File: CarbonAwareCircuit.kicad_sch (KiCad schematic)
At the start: 3 parts, among them J1 USB_C_Receptacle_PowerOnly_6P, U1 LD1117V33, U2 ESP32-C3

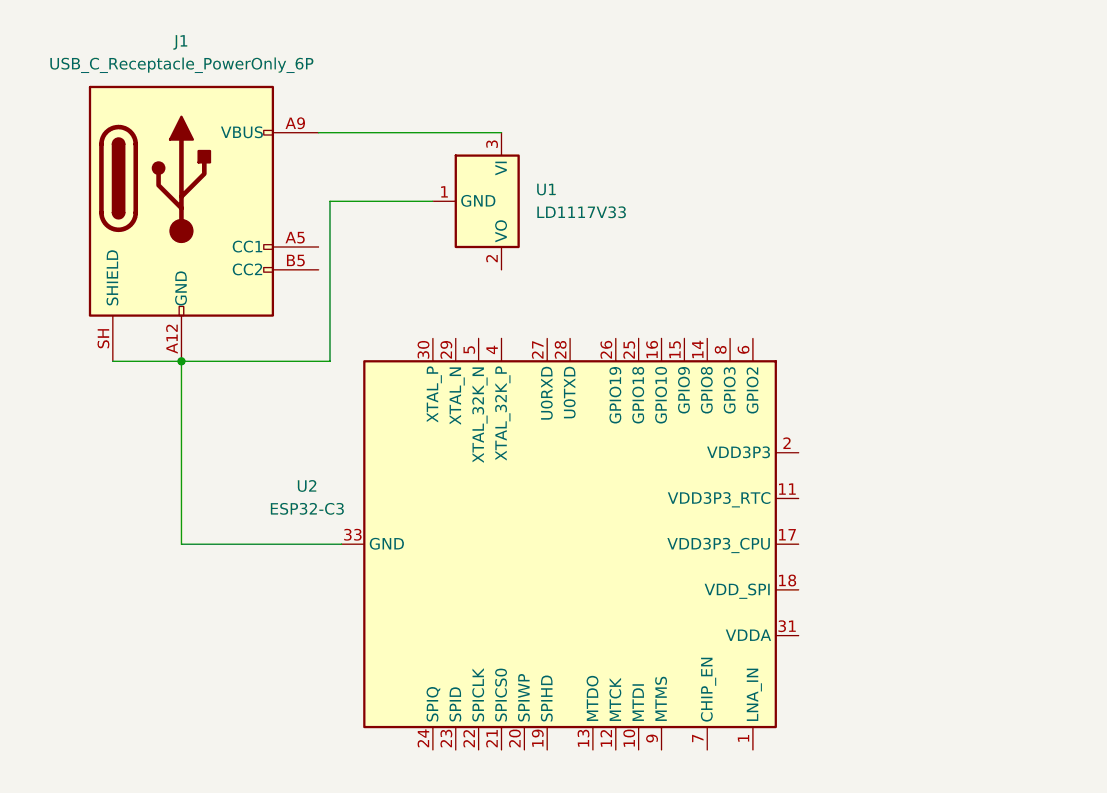
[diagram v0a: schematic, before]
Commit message: more circuit tweaks
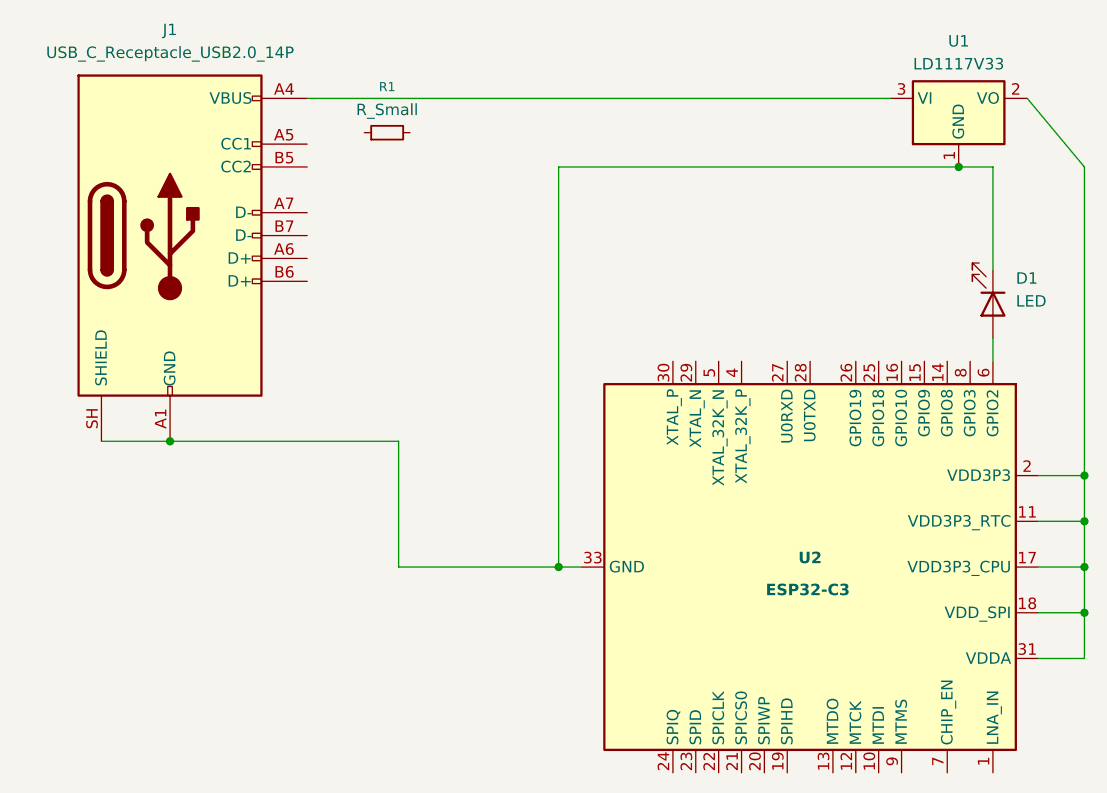
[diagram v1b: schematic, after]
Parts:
- removed J1: USB_C_Receptacle_PowerOnly_6P, symbol Connector:USB_C_Receptacle_PowerOnly_6P
- added D1: LED, symbol Device:LED
- added J1: USB_C_Receptacle_USB2.0_14P, symbol Connector:USB_C_Receptacle_USB2.0_14P
- added R1: R_Small, symbol Device:R_Small
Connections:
- net at U2.11 (VDD3P3_RTC): now also U1.2 (VO), U2.17 (VDD3P3_CPU), U2.18 (VDD_SPI), U2.2 (VDD3P3), U2.3 (VDD3P3), U2.31 (VDDA), U2.32 (VDDA)
- net at U1.1 (GND), U2.33 (GND): now also D1.1 (K), J1.A1 (GND), J1.A12 (GND), J1.B1 (GND), J1.B12 (GND), J1.SH (SHIELD)
- net at U2.6 (GPIO2): now also D1.2 (A)
- net at U1.3 (VI): now also J1.A4 (VBUS), J1.A9 (VBUS), J1.B4 (VBUS), J1.B9 (VBUS)
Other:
- moved on the sheet: U1, U2
